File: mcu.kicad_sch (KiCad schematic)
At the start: 23 parts, among them U1 SF32LB525UC6, U2 GD25Q256EWIGR, Y1 48MHz, Y2 32.768khz

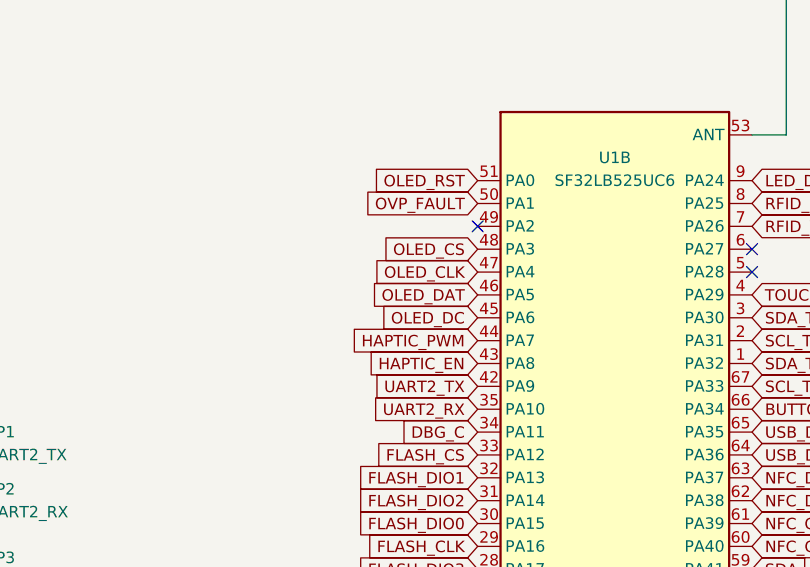
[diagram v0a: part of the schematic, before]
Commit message: first draft of final board
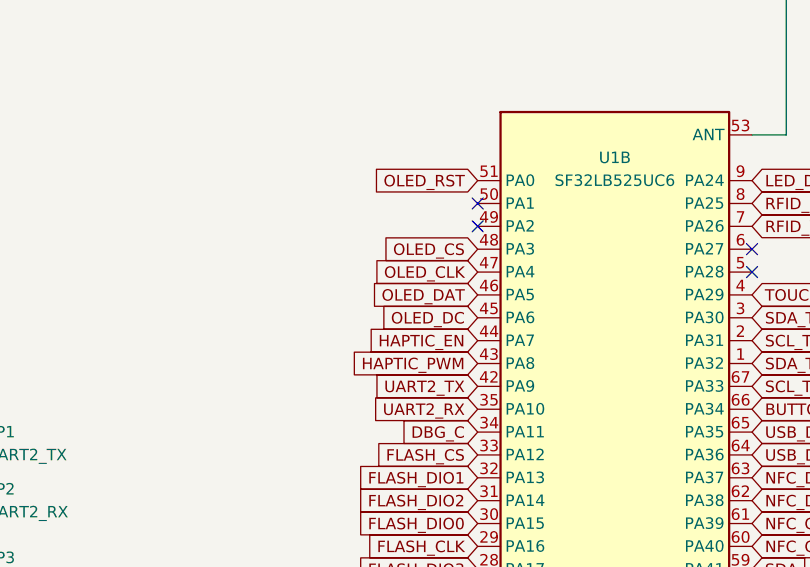
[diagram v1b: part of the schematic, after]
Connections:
- net HAPTIC_EN: now also U1.44 (PA7); no longer U1.43 (PA8)
- net HAPTIC_PWM: now also U1.43 (PA8); no longer U1.44 (PA7)
- net OVP_FAULT: no longer names the net of U1.50 (PA1)
- no-connect marks 9 -> 10

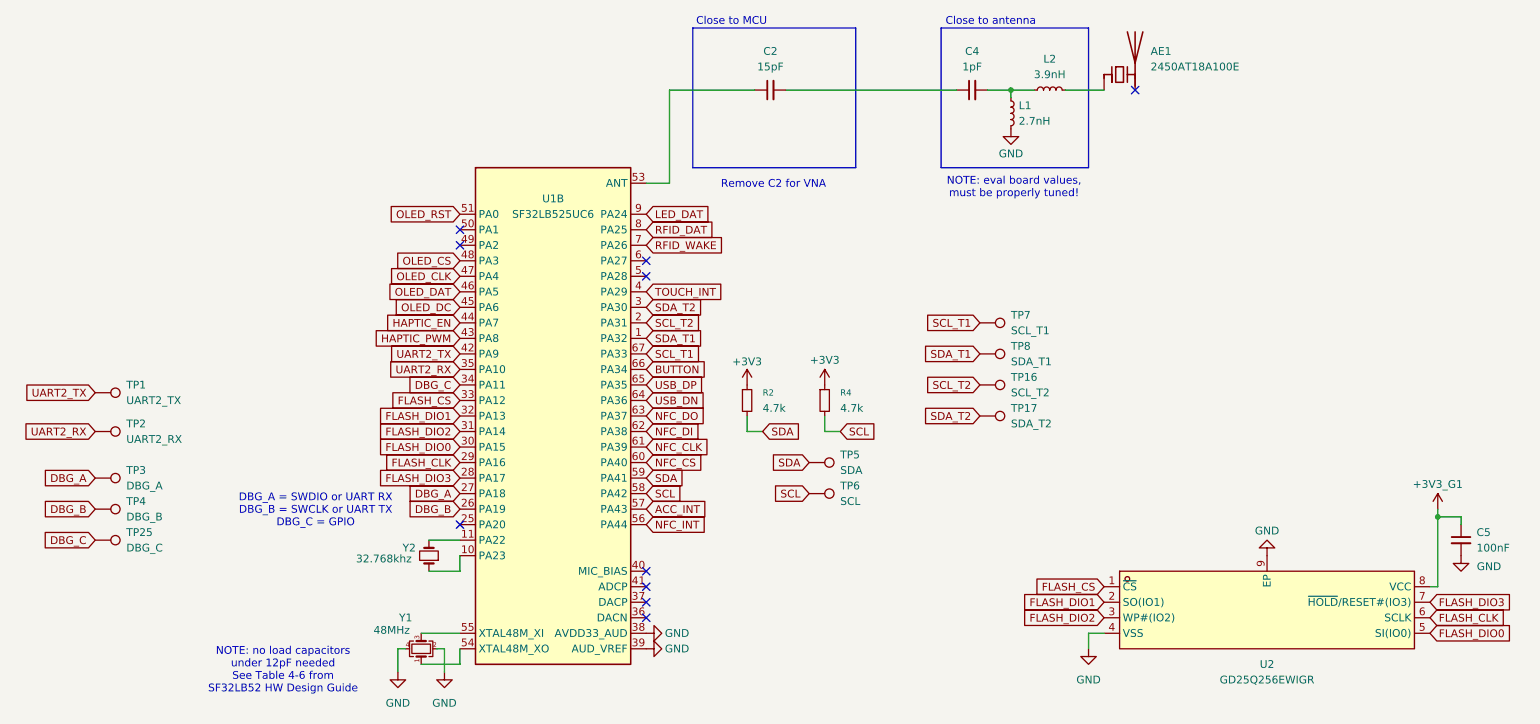
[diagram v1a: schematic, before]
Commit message: final fixups before prod
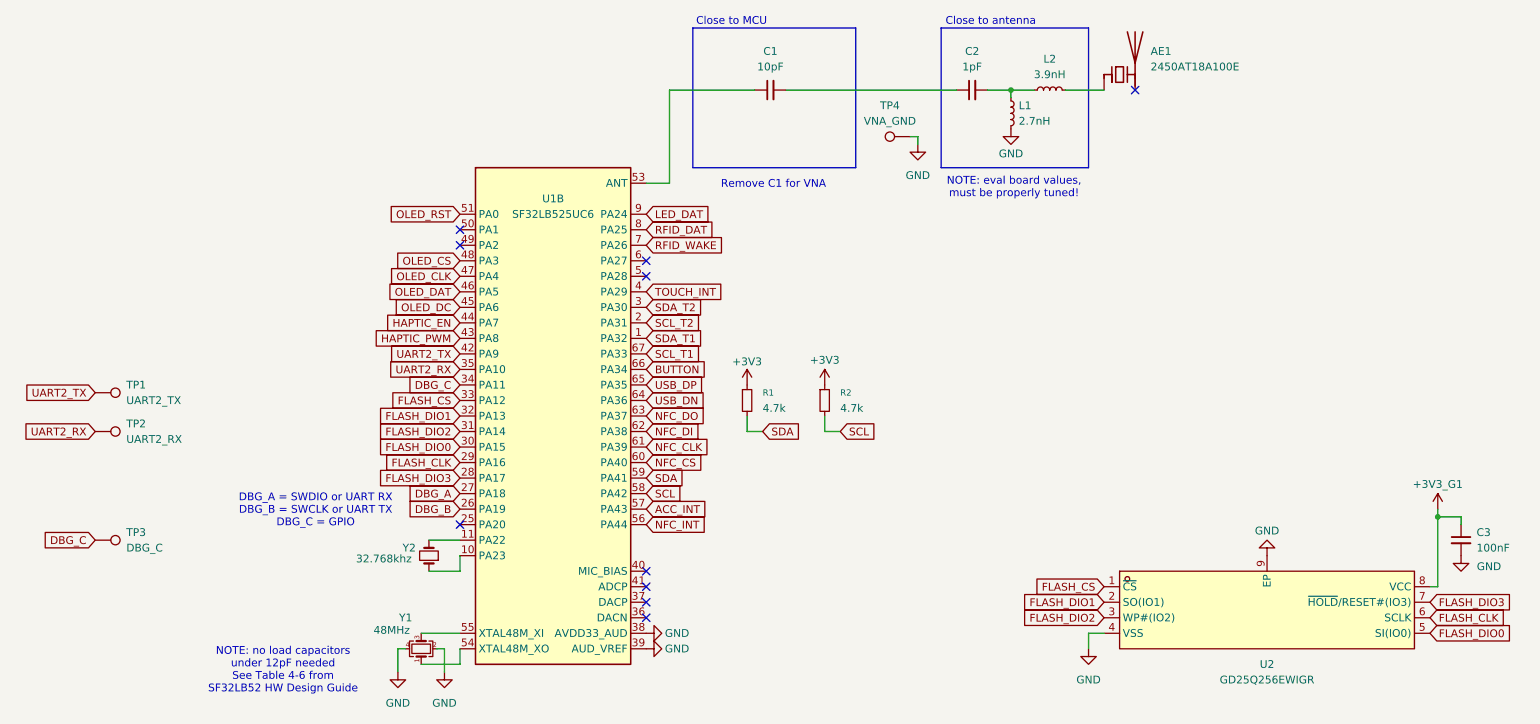
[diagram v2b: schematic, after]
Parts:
- removed TP16: SCL_T2, TestPoint:TestPoint_Pad_D1.0mm, symbol Connector:TestPoint
- removed TP17: SDA_T2, TestPoint:TestPoint_Pad_D1.0mm, symbol Connector:TestPoint
- removed TP3: DBG_A, TestPoint:TestPoint_Pad_D1.0mm, symbol Connector:TestPoint
- removed TP5: SDA, TestPoint:TestPoint_Pad_D1.0mm, symbol Connector:TestPoint
- removed TP6: SCL, TestPoint:TestPoint_Pad_D1.0mm, symbol Connector:TestPoint
- removed TP7: SCL_T1, TestPoint:TestPoint_Pad_D1.0mm, symbol Connector:TestPoint
- removed TP8: SDA_T1, TestPoint:TestPoint_Pad_D1.0mm, symbol Connector:TestPoint
- C1: renamed from C2; value 15pF -> 10pF; LCSC Part C1548 -> C32949
- C2: renamed from C4; LCSC Part C37117 -> C307493
- TP4: value DBG_B -> VNA_GND
- renumbered C5 to C3, R2 to R1, R4 to R2, TP25 to TP3
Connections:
- net DBG_B: no longer TP4.1
- net GND: now also TP4.1
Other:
- note added: "Remove C1 for VNA"
- note removed: "Remove C2 for VNA"
